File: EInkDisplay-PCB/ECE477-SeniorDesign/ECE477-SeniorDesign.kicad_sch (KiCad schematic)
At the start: 5 parts

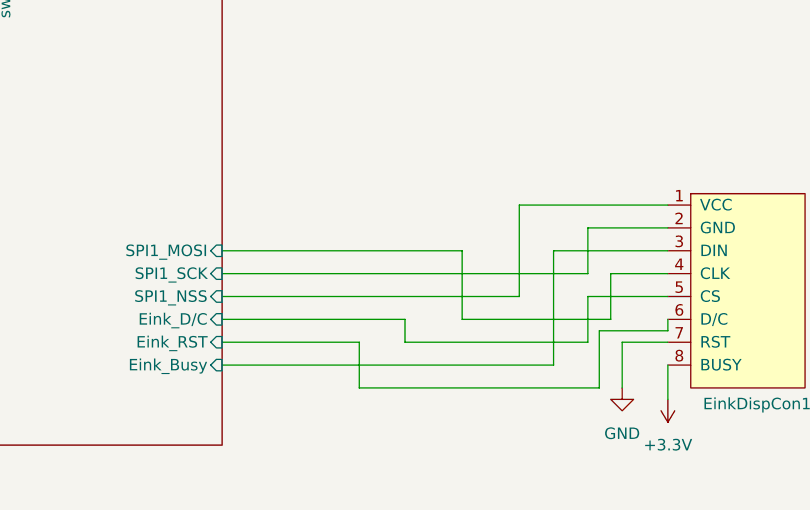
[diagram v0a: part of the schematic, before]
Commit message: push
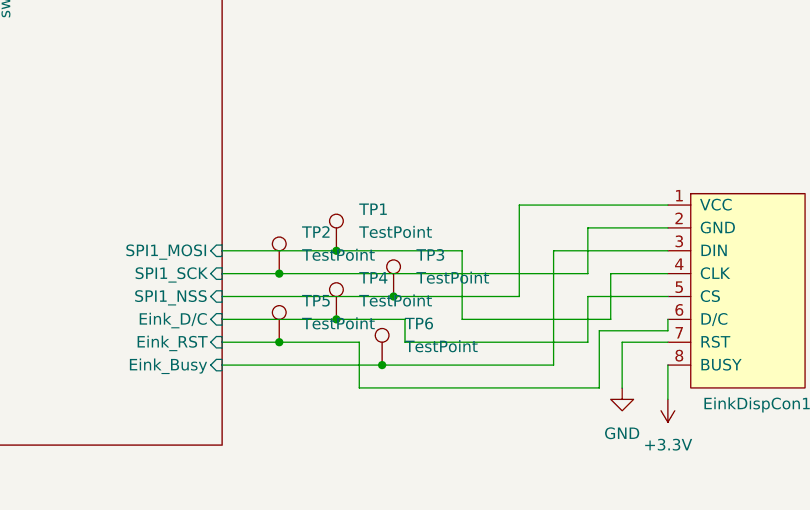
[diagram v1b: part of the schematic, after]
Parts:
- added TP1, TP2, TP3, TP4, TP5, TP6: TestPoint, TestPoint:TestPoint_Pad_D2.0mm, symbol Connector:TestPoint
- EinkDispCon1: footprint Connector_PinHeader_1.00mm:PinHeader_1x08_P1.00mm_Vertical -> Connector_PinHeader_2.54mm:PinHeader_1x08_P2.54mm_Vertical
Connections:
- net MCU/Eink_Busy: now also TP6.1
- net MCU/Eink_D/C: now also TP4.1
- net MCU/Eink_RST: now also TP5.1
- net MCU/SPI1_MOSI: now also TP1.1
- net MCU/SPI1_NSS: now also TP3.1
- net MCU/SPI1_SCK: now also TP2.1
